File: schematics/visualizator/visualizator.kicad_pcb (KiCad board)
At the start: 2 copper layers, 39.3 x 43.2 mm, 20 parts, among them J1 5V, J2 WS2812, J3 Audio, SW1 COLOR, SW2 PATTERN, U1 ATmega328-16PU, Y1 16MHz

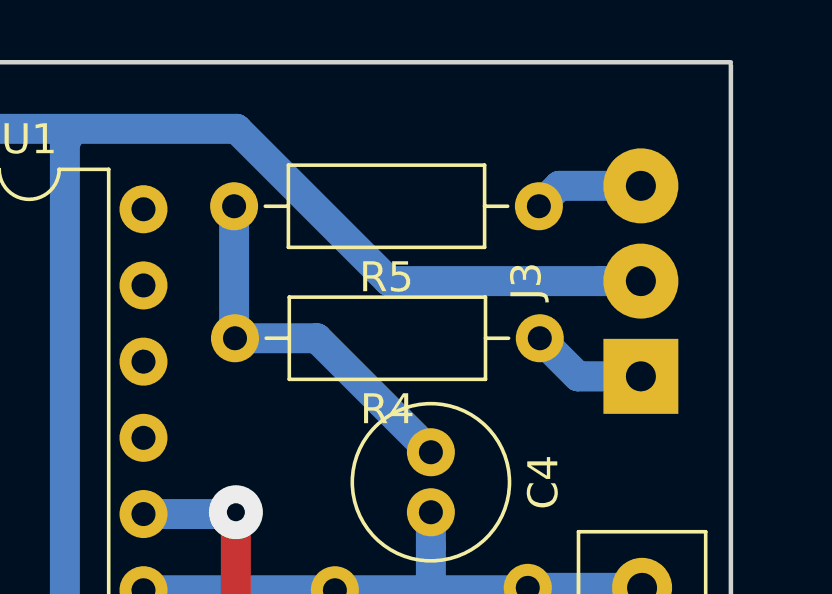
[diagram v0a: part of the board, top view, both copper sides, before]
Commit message: PCB updated
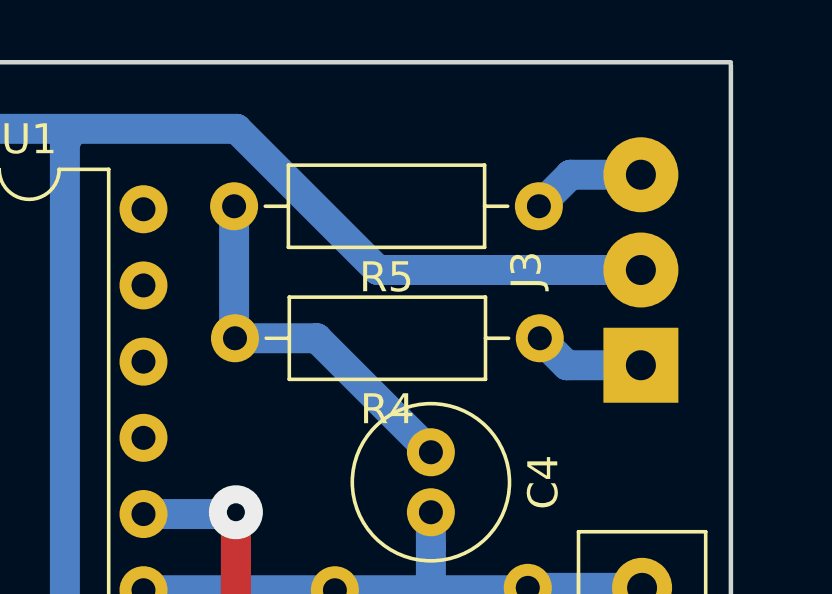
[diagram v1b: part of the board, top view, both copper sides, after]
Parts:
- moved J3 0.37 mm to (90.3, 40.6)
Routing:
- net Net-(C1-Pad1): track 141.7 -> 141.1 mm
- net Net-(J3-Pad1): track 4.34 -> 3.74 mm
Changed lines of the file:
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@@
     (thickness 1.6)
     (drawings 6)
-    (tracks 108)
+    (tracks 107)
     (zones 0)
     (modules 20)
@@
   )
   (module Connector_Wire:SolderWirePad_1x03_P3.175mm_Drill1mm (layer F.Cu)
-    (at 90.3 40.97 90)
+    (at 90.3 40.6 90)
     (descr "Wire solder connection")
     (tags connector)
@@
   (segment (start 90.34 58.02) (end 90.34 64.61) (width 1) (layer B.Cu) (net 13))
   (segment (start 55.88 35.26) (end 58.42 32.72) (width 1) (layer B.Cu) (net 13))
-  (segment (start 88.972686 37.795) (end 90.74 37.795) (width 1) (layer B.Cu) (net 13))
-  (segment (start 81.899002 37.795) (end 88.972686 37.795) (width 1) (layer B.Cu) (net 13))
-  (segment (start 76.824002 32.72) (end 81.899002 37.795) (width 1) (layer B.Cu) (net 13))
   (segment (start 58.42 32.72) (end 76.824002 32.72) (width 1) (layer B.Cu) (net 13))
   (segment (start 83.3 54.95) (end 86.53 58.18) (width 1) (layer B.Cu) (net 13))
@@
   (segment (start 64.96863 53.18) (end 63.18863 51.4) (width 1) (layer B.Cu) (net 13))
   (segment (start 63.18863 44.798628) (end 57.890002 39.5) (width 1) (layer B.Cu) (net 13))
+  (segment (start 81.529002 37.425) (end 90.3 37.425) (width 1) (layer B.Cu) (net 13))
+  (segment (start 76.824002 32.72) (end 81.529002 37.425) (width 1) (layer B.Cu) (net 13))
   (segment (start 60.8 45) (end 60.8 51.6) (width 1) (layer B.Cu) (net 14))
   (segment (start 57.6 41.8) (end 60.8 45) (width 1) (layer B.Cu) (net 14))
@@
   (segment (start 76.74 39.67) (end 76.77 39.7) (width 1) (layer B.Cu) (net 26))
   (segment (start 76.74 35.3) (end 76.74 39.67) (width 1) (layer B.Cu) (net 26))
-  (segment (start 87.58 34.62) (end 86.9 35.3) (width 1) (layer B.Cu) (net 27))
-  (segment (start 90.74 34.62) (end 87.58 34.62) (width 1) (layer B.Cu) (net 27))
-  (segment (start 88.2 40.97) (end 86.93 39.7) (width 1) (layer B.Cu) (net 28))
-  (segment (start 90.74 40.97) (end 88.2 40.97) (width 1) (layer B.Cu) (net 28))
+  (segment (start 87.95 34.25) (end 86.9 35.3) (width 1) (layer B.Cu) (net 27))
+  (segment (start 90.3 34.25) (end 87.95 34.25) (width 1) (layer B.Cu) (net 27))
+  (segment (start 87.83 40.6) (end 86.93 39.7) (width 1) (layer B.Cu) (net 28))
+  (segment (start 90.3 40.6) (end 87.83 40.6) (width 1) (layer B.Cu) (net 28))
   (segment (start 81.886508 67.945) (end 83.3 67.945) (width 1) (layer B.Cu) (net 29))
   (segment (start 80.1 58.26) (end 80.1 66.158492) (width 1) (layer B.Cu) (net 29))
